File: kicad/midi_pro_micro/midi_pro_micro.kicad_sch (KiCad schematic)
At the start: 4 parts, among them J1 DIN-5_180degree, J2 DIN-5_180degree, U1 ProMicro

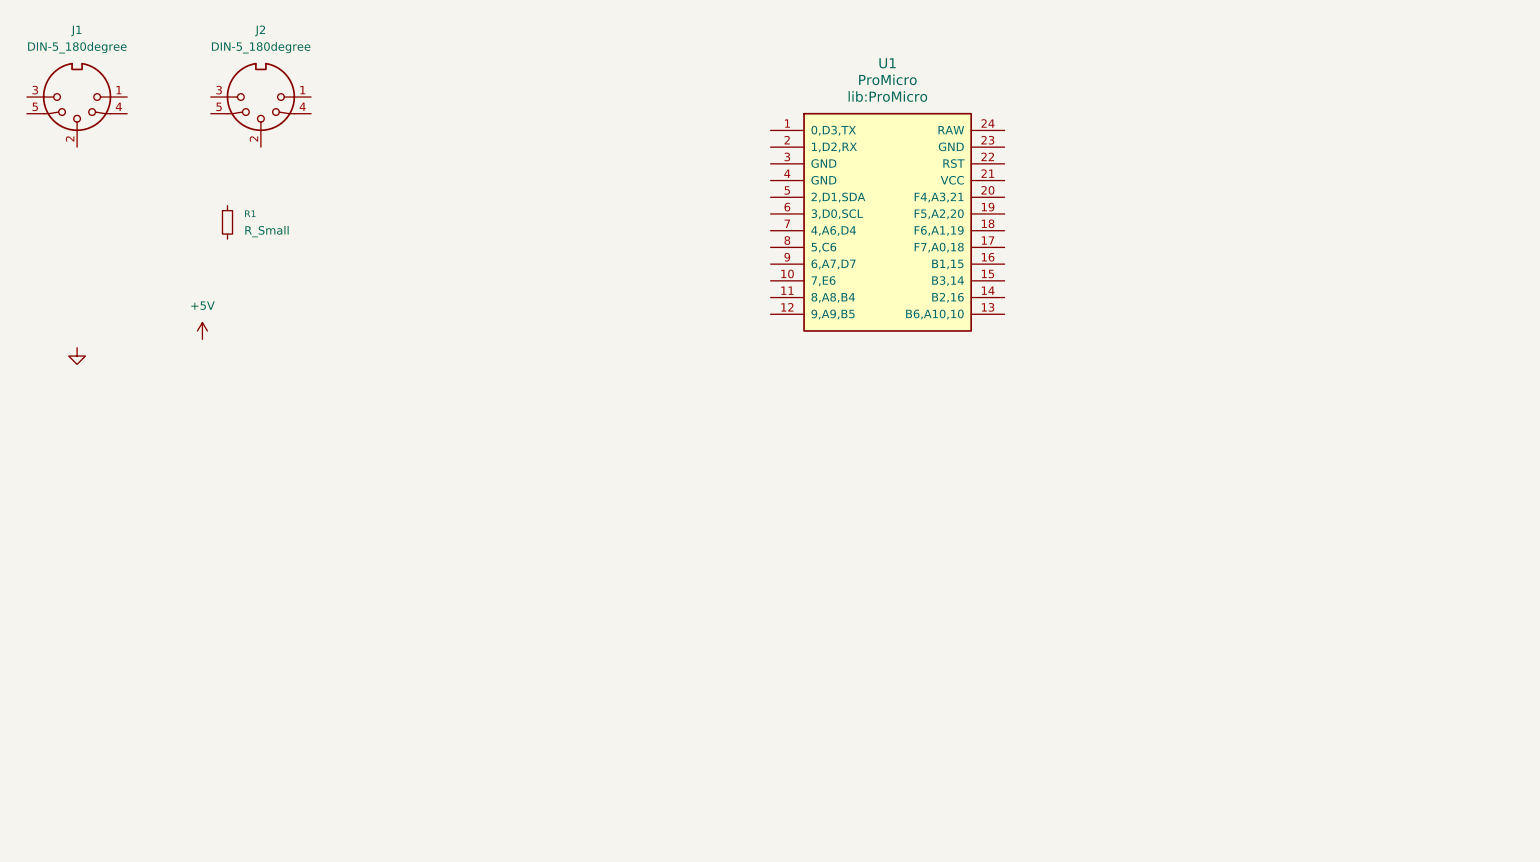
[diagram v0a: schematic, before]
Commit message: Draft schematic
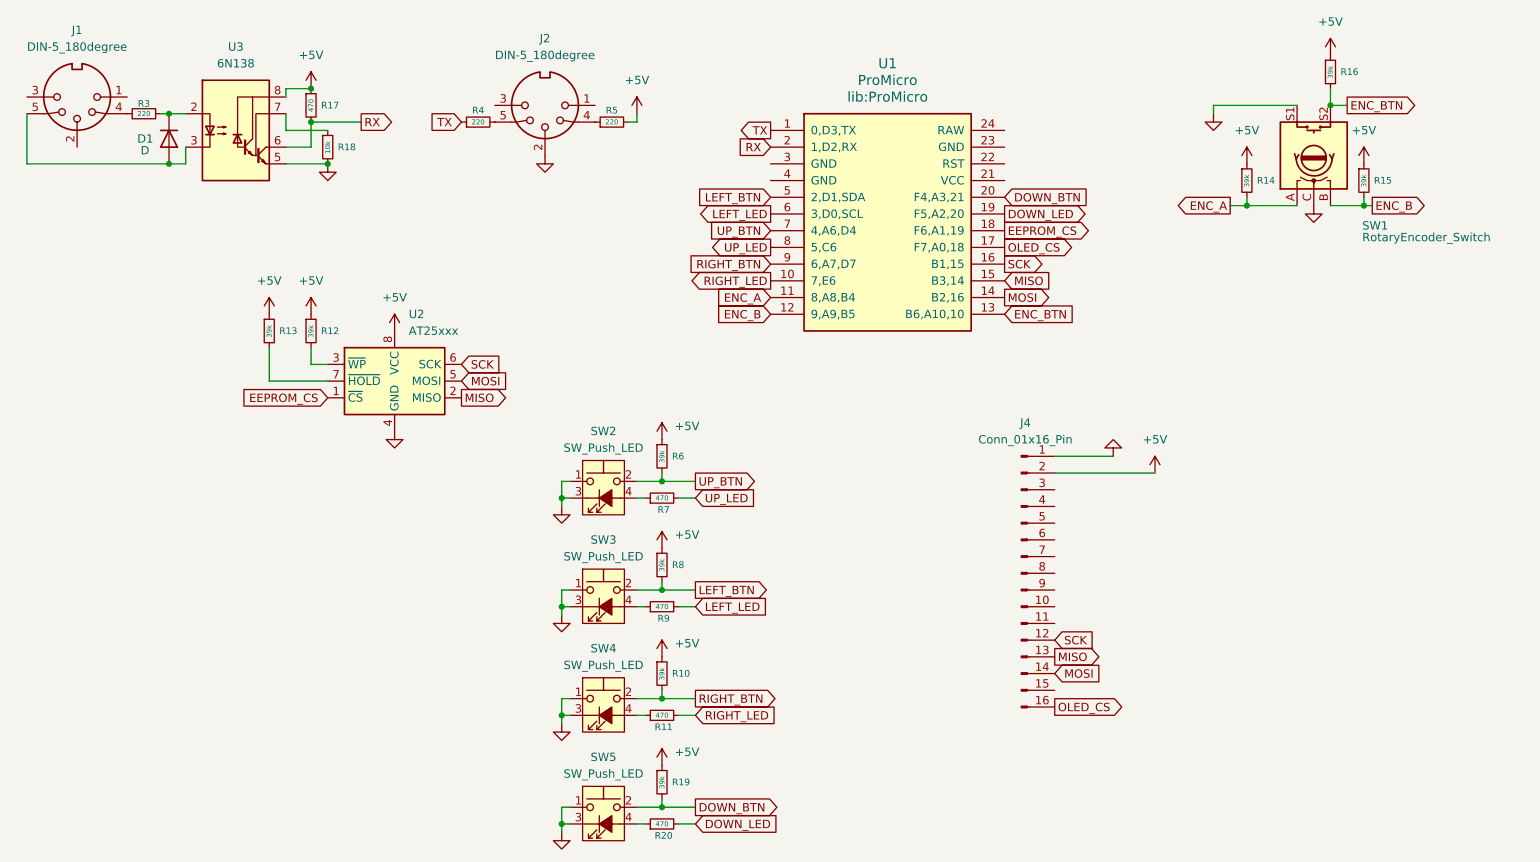
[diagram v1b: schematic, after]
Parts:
- removed R1: R_Small, Resistor_SMD:R_0805_2012Metric_Pad1.20x1.40mm_HandSolder, symbol Device:R_Small
- added D1: D, symbol Device:D
- added J4: Conn_01x16_Pin, Connector_PinHeader_2.54mm:PinHeader_1x16_P2.54mm_Vertical, symbol Connector:Conn_01x16_Pin
- added R10, R12, R13, R14, R15, R16, R19, R6, R8: 39k, Resistor_SMD:R_0805_2012Metric_Pad1.20x1.40mm_HandSolder, symbol Device:R_Small
- added R11, R17, R20, R7, R9: 470, Resistor_SMD:R_0805_2012Metric_Pad1.20x1.40mm_HandSolder, symbol Device:R_Small
- added R18: 10k, Resistor_SMD:R_0805_2012Metric_Pad1.20x1.40mm_HandSolder, symbol Device:R_Small
- added R3, R4, R5: 220, Resistor_SMD:R_0805_2012Metric_Pad1.20x1.40mm_HandSolder, symbol Device:R_Small
- added SW1: RotaryEncoder_Switch, Rotary_Encoder:RotaryEncoder_Bourns_Vertical_PEC12R-3x17F-Sxxxx, symbol Device:RotaryEncoder_Switch
- added SW2, SW3, SW4, SW5: SW_Push_LED, lib:SW_PUSH_6mm, symbol Switch:SW_Push_LED
- added U2: AT25xxx, symbol Memory_EEPROM:AT25xxx
- added U3: 6N138, symbol Isolator:6N138
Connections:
- net +5V: now also J4.2 (Pin_2), R10.1, R12.1, R13.1, R14.1, R15.1, R16.1, R17.1, R19.1, R5.2, R6.1, R8.1, U2.8 (VCC), U3.8 (VCC)
- net GND: now also J2.2, J4.1 (Pin_1), R18.2, SW1.C, SW1.S1, SW2.1, SW2.3 (K), SW3.1, SW3.3 (K), SW4.1, SW4.3 (K), SW5.1, SW5.3 (K), U2.4 (GND), U3.5 (GND)
- net at J1.4: now also R3.1
- net at J1.5: now also D1.2 (A), U3.3 (C2)
- net TX: now reaches U1.1 (0,D3,TX)
- net TX: now also R4.1
- net RIGHT_LED: now reaches U1.10 (7,E6)
- net RIGHT_LED: now also R11.2
- net ENC_A: now reaches U1.11 (8,A8,B4)
- net ENC_A: now also R14.2, SW1.A
- net ENC_B: now reaches U1.12 (9,A9,B5)
- net ENC_B: now also R15.2, SW1.B
- net ENC_BTN: now reaches U1.13 (B6,A10,10)
- net ENC_BTN: now also R16.2, SW1.S2
- net MOSI: now reaches U1.14 (B2,16)
- net MOSI: now also J4.14 (Pin_14), U2.5 (MOSI)
- net MISO: now reaches U1.15 (B3,14)
- net MISO: now also J4.13 (Pin_13), U2.2 (MISO)
- net SCK: now reaches U1.16 (B1,15)
- net SCK: now also J4.12 (Pin_12), U2.6 (SCK)
- net OLED_CS: now reaches U1.17 (F7,A0,18)
- net OLED_CS: now also J4.16 (Pin_16)
- net EEPROM_CS: now reaches U1.18 (F6,A1,19)
- net EEPROM_CS: now also U2.1 (~{CS})
- net DOWN_LED: now reaches U1.19 (F5,A2,20)
- net DOWN_LED: now also R20.2
- net RX: now reaches U1.2 (1,D2,RX)
- net RX: now also R17.2, U3.6 (VO2)
- net DOWN_BTN: now reaches U1.20 (F4,A3,21)
- net DOWN_BTN: now also R19.2, SW5.2
- net LEFT_BTN: now reaches U1.5 (2,D1,SDA)
- net LEFT_BTN: now also R8.2, SW3.2
- net LEFT_LED: now reaches U1.6 (3,D0,SCL)
- net LEFT_LED: now also R9.2
- net UP_BTN: now reaches U1.7 (4,A6,D4)
- net UP_BTN: now also R6.2, SW2.2
- net UP_LED: now reaches U1.8 (5,C6)
- net UP_LED: now also R7.2
- net RIGHT_BTN: now reaches U1.9 (6,A7,D7)
- net RIGHT_BTN: now also R10.2, SW4.2
- net at J2.4: now also R5.1
- net at J2.5: now also R4.2
- new net: R11.1, SW4.4 (A)
- new net: R20.1, SW5.4 (A)
- new net: R18.1, U3.7 (VO1)
- new net: D1.1 (K), R3.2, U3.2 (C1)
- new net: R12.2, U2.3 (~{WP})
- new net: R13.2, U2.7 (~{HOLD})
- new net: R7.1, SW2.4 (A)
- new net: R9.1, SW3.4 (A)
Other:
- moved on the sheet: J2
